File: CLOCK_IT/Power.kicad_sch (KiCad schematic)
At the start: 39 parts, among them J17 Conn_01x04_Socket, Q3 AO3400A, Q4 AO3400A, U19 DS1307N+, U4 AXP2101, Y2 32.768kHz

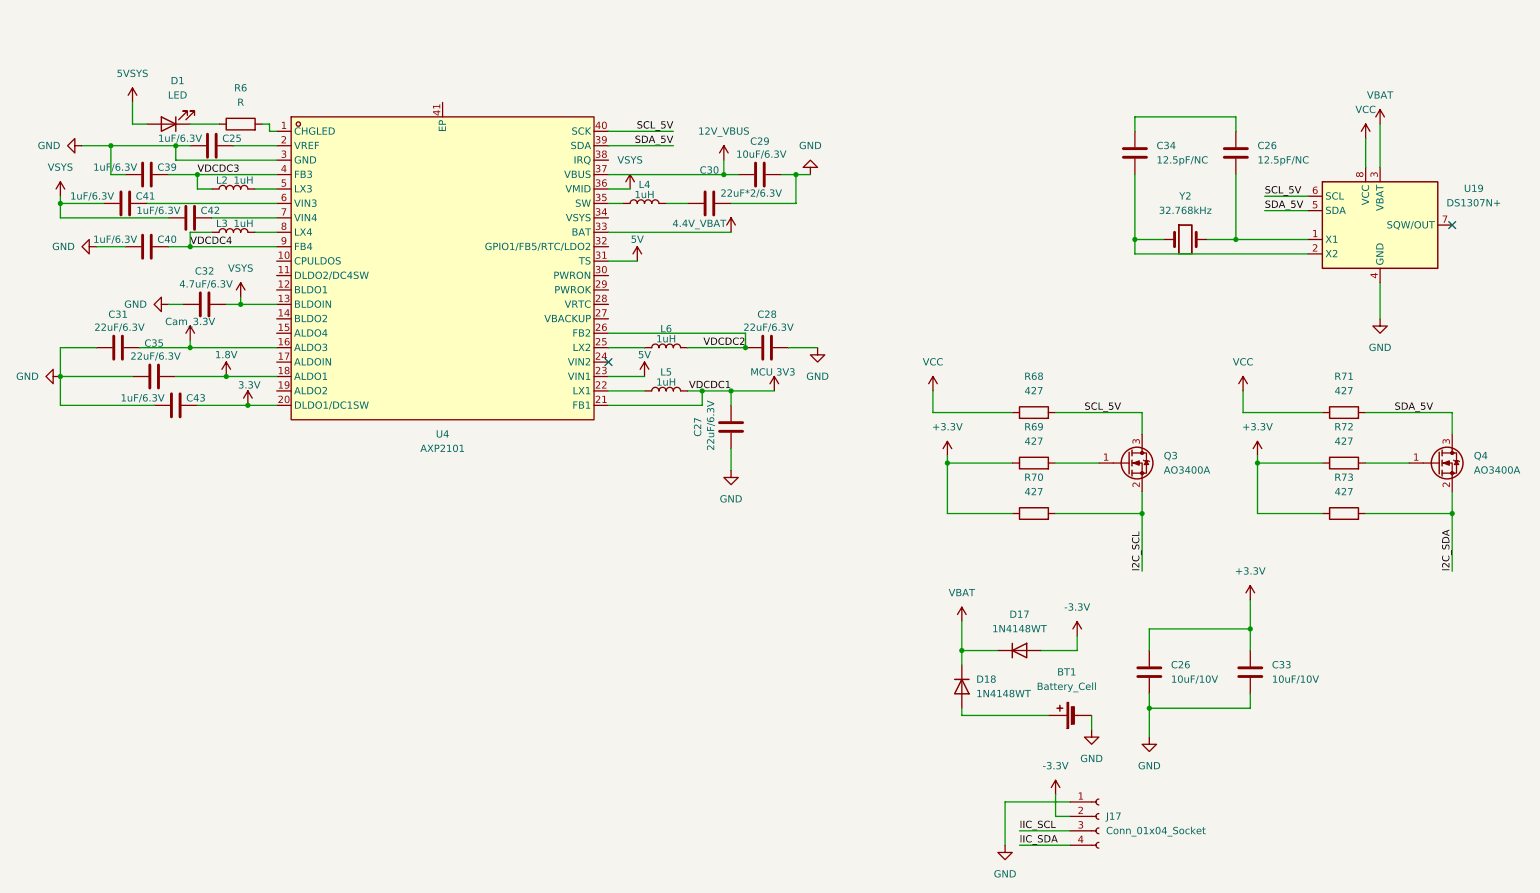
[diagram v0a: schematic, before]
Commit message: :fire: WORKING ON POWER
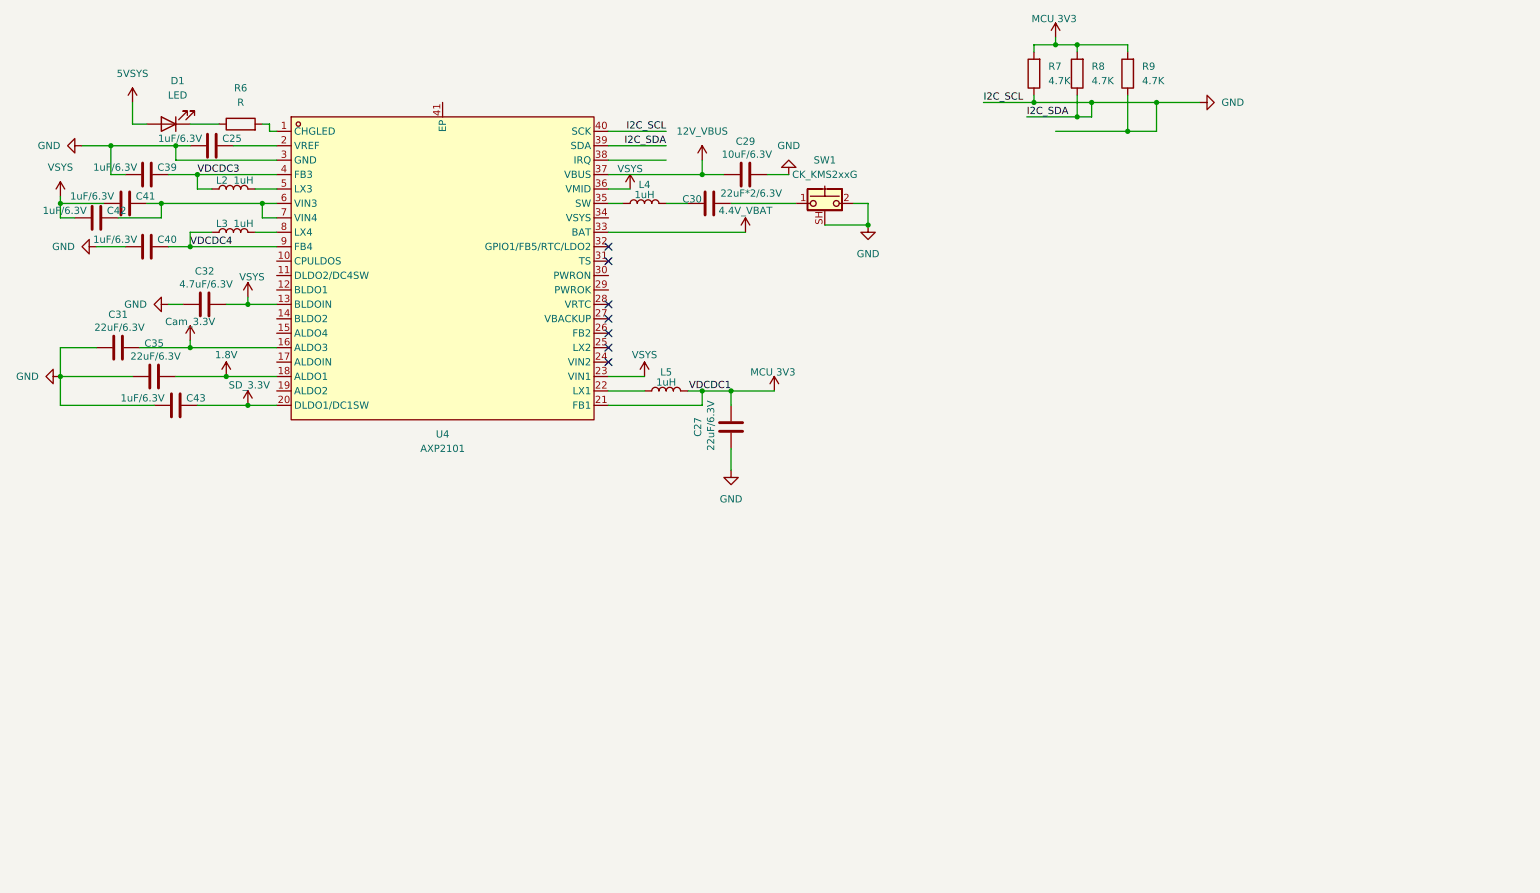
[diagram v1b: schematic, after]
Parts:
- removed BT1: Battery_Cell, Battery:BatteryHolder_MPD_BH-18650-PC2, symbol Device:Battery_Cell
- removed C26, C33: 10uF/10V, Capacitor_Tantalum_SMD:CP_EIA-2012-12_Kemet-R, symbol Device:C
- removed C26, C34: 12.5pF/NC, Capacitor_Tantalum_SMD:CP_EIA-2012-12_Kemet-R, symbol Device:C
- removed C28: 22uF/6.3V, symbol Device:C
- removed D17, D18: 1N4148WT, Diode_SMD:D_SOD-523, symbol Diode:1N4148WT
- removed J17: Conn_01x04_Socket, Module:Flipper_Zero_Angled, symbol Connector:Conn_01x04_Socket
- removed L6: 1uH, symbol Device:L
- removed Q3, Q4: AO3400A, Package_TO_SOT_SMD:SOT-23, symbol Transistor_FET:AO3400A
- removed R68, R69, R70, R71, R72, R73: 427, Resistor_SMD:R_01005_0402Metric_Pad0.57x0.30mm_HandSolder, symbol Device:R
- removed U19: DS1307N+, Package_DIP:DIP-8_W7.62mm, symbol Timer_RTC:DS1307N+
- removed Y2: 32.768kHz, Oscillator:Oscillator_SMD_Fox_FT5H_5.0x3.2mm, symbol Device:Crystal
- added R7, R8, R9: 4.7K, symbol Device:R
- added SW1: CK_KMS2xxG, Button_Switch_SMD:SW_SPST_CK_KMS2xxGP, symbol Switch:CK_KMS2xxG
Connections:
- net SCL_5V is gone; now on net GND: U4.40 (SCK)
- net SDA_5V is gone; now on net GND: U4.39 (SDA)
- net GND: now also R7.1, R8.1, R9.1, SW1.2, SW1.SH (B); no longer C30.2
- net MCU 3V3: now also R7.2, R8.2, R9.2
- net VSYS: now also U4.23 (VIN1)
- net at C41.2, U4.6 (VIN3): now also C42.2, U4.7 (VIN4)
- net 3.3V renamed SD_3.3V
- net 5V: no longer names the net of U4.31 (TS)
- net 5V: no longer U4.23 (VIN1)
- net VDCDC2: no longer names the net of U4.26 (FB2)
- new net: C30.2, SW1.1
- no-connect marks 2 -> 7
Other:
- moved on the sheet: C29, C42
